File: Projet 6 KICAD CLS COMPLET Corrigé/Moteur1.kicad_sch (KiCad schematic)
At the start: 16 parts

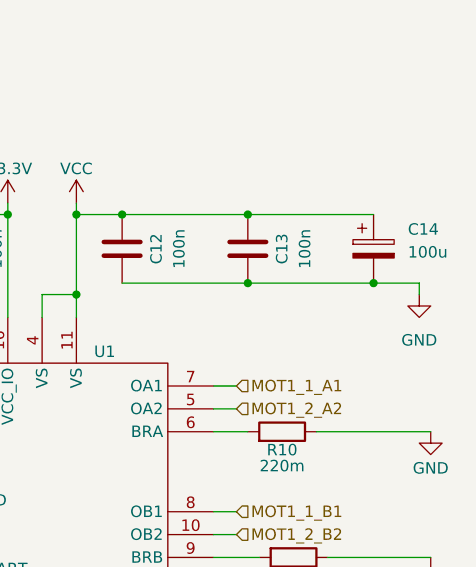
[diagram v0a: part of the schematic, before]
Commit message: Add files via upload
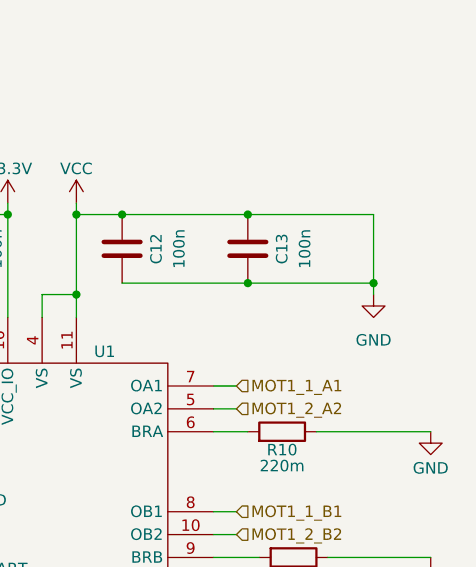
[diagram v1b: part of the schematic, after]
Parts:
- removed C14: 100u, symbol Device:C_Polarized
- C12, C13, C15, C22, C23, C3: footprint (none) -> Capacitor_SMD:C_0805_2012Metric
- D2: footprint (none) -> LED_SMD:LED_0603_1608Metric
- R10, R11: footprint (none) -> Resistor_SMD:R_1206_3216Metric
- R12, R15, R16, R8, R9: footprint (none) -> Resistor_SMD:R_0603_1608Metric
- U1: footprint (none) -> Package_SO:HTSSOP-28-1EP_4.4x9.7mm_P0.65mm_EP2.85x5.4mm_ThermalVias
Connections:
- net VCC is gone; now on net GND: C12.1, C13.1, C22.2, U1.11 (VS), U1.4 (VS)
